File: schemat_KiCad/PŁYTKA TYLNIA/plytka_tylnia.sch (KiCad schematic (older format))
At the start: 48 parts, among them P1 USB_OTG, SW1 SPST

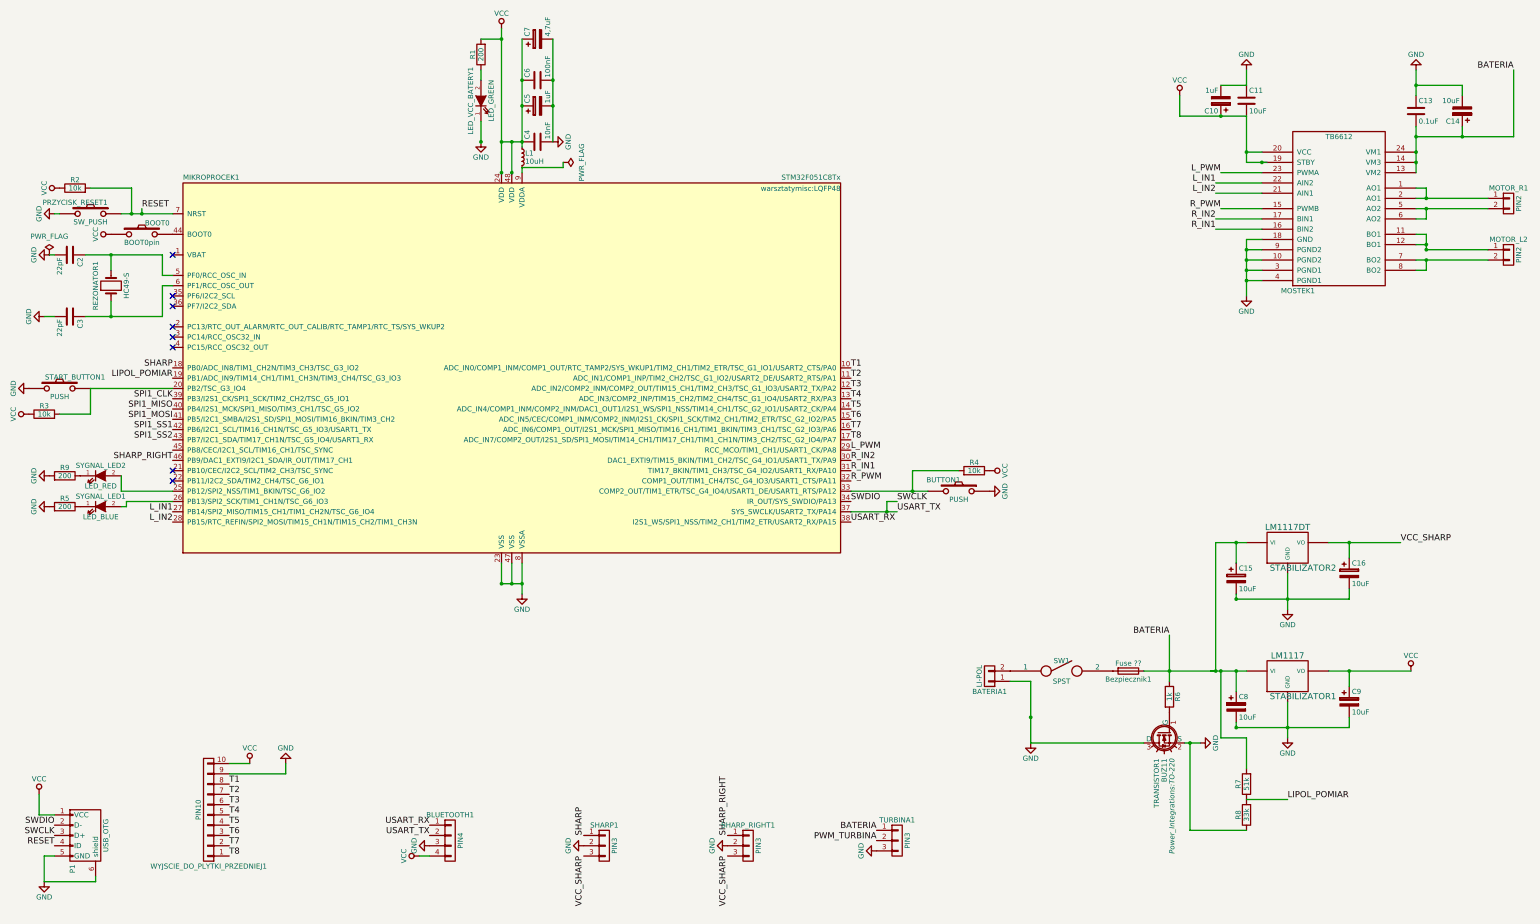
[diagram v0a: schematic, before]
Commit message: zrobiony przełącznik boot0
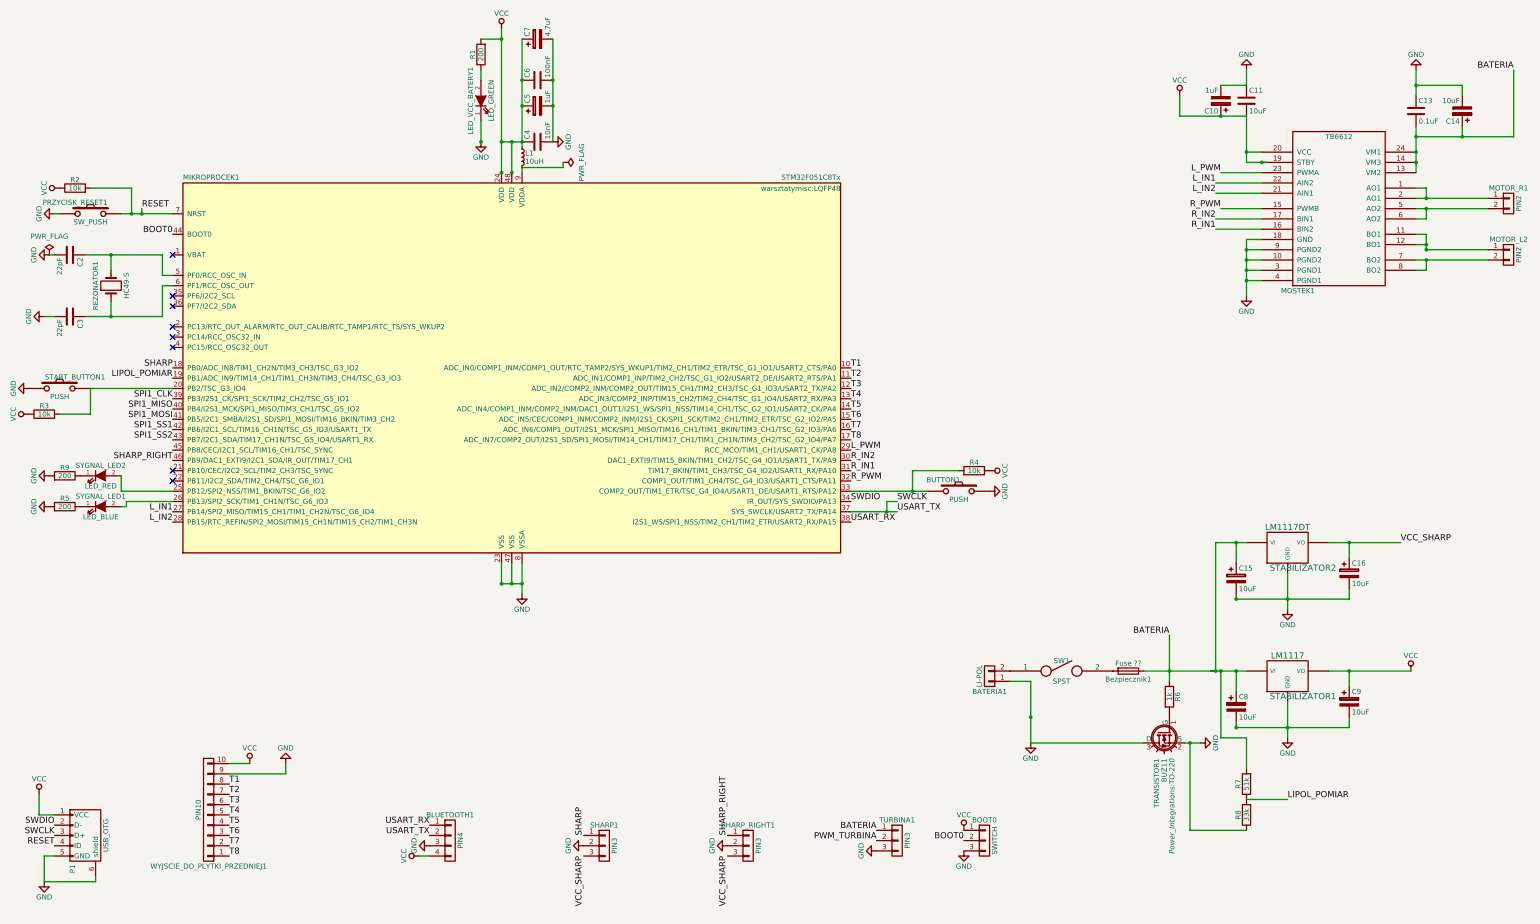
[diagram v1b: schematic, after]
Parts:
- removed BOOT0: BOOT0pin, symbol SW_PUSH
- added BOOT0: SWITCH, symbol CONN_01X03
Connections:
- net GND: now also BOOT0.3 (P3)
- net VCC: now also BOOT0.1 (P1)
- net BOOT0: now reaches MIKROPROCEK1.44 (BOOT0)
- net BOOT0: now also BOOT0.2 (P2)
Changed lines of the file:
@@
 SHARP
-$Comp
-L SW_PUSH BOOT0
-U 1 1 58DBFC59
-P 2300 3200
-F 0 "BOOT0" H 2450 3310 50  0000 C CNN
-F 1 "BOOT0pin" H 2300 3120 50  0000 C CNN
-F 2 "" H 2300 3200 50  0000 C CNN
-F 3 "" H 2300 3200 50  0000 C CNN
-	1    2300 3200
-	1    0    0    -1
-$EndComp
-$Comp
-L VCC #PWR11
-U 1 1 58DBFCD6
-P 2000 3200
-F 0 "#PWR11" H 2000 3050 50  0001 C CNN
-F 1 "VCC" H 2000 3350 50  0000 C CNN
-F 2 "" H 2000 3200 50  0001 C CNN
-F 3 "" H 2000 3200 50  0001 C CNN
-	1    2000 3200
-	0    -1   -1   0
-$EndComp
 $Comp
 L STM32F051C8Tx MIKROPROCEK1
@@
 	0    1    1    0
 $EndComp
+Text Label 2600 3200 2    60   ~ 0
+BOOT0
+Text Label 10300 9100 2    60   ~ 0
+BOOT0
+$Comp
+L VCC #PWR?
+U 1 1 58E56396
+P 10300 9000
+F 0 "#PWR?" H 10300 8850 50  0001 C CNN
+F 1 "VCC" H 10300 9150 50  0000 C CNN
+F 2 "" H 10300 9000 50  0001 C CNN
+F 3 "" H 10300 9000 50  0001 C CNN
+	1    10300 9000
+	1    0    0    -1
+$EndComp
+$Comp
+L CONN_01X03 BOOT0
+U 1 1 58E56485
+P 10500 9100
+F 0 "BOOT0" H 10500 9300 50  0000 C CNN
+F 1 "SWITCH" V 10600 9100 50  0000 C CNN
+F 2 "" H 10500 9100 50  0001 C CNN
+F 3 "" H 10500 9100 50  0001 C CNN
+	1    10500 9100
+	1    0    0    -1
+$EndComp
+$Comp
+L GND #PWR?
+U 1 1 58E56822
+P 10300 9200
+F 0 "#PWR?" H 10300 8950 50  0001 C CNN
+F 1 "GND" H 10300 9050 50  0000 C CNN
+F 2 "" H 10300 9200 50  0001 C CNN
+F 3 "" H 10300 9200 50  0001 C CNN
+	1    10300 9200
+	1    0    0    -1
+$EndComp
 $EndSCHEMATC
